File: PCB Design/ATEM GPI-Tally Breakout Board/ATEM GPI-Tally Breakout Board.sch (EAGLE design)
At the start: 22 parts, among them X1 DB25M

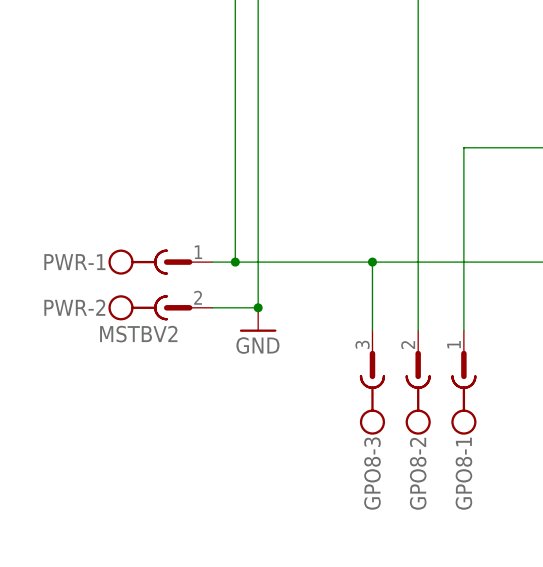
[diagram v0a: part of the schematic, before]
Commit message: Updates for PCBs and more
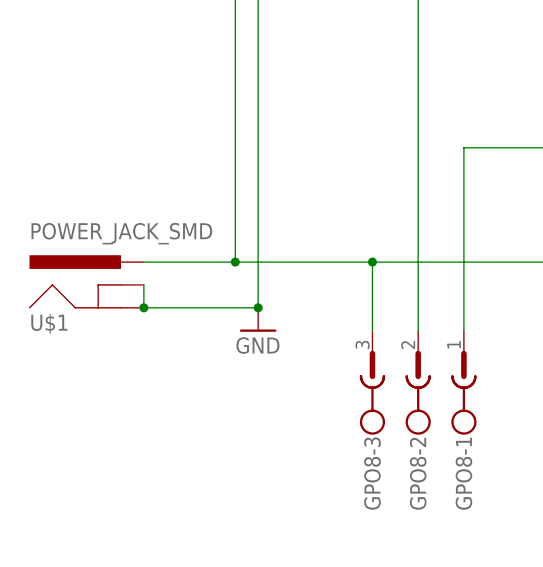
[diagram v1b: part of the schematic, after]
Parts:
- removed PWR: MSTBV2, con-phoenix-508:MSTBV2
- added U$1: POWER_JACK_SMD, SKAARHOJ:POWER_JACK_SMD
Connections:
- net GND: now also U$1.GND, U$1.GNDBREAK; no longer PWR-2.1
- net N$75: now also U$1.PWR; no longer PWR-1.1
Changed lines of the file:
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@@
 <?xml version="1.0" encoding="utf-8"?>
 <!DOCTYPE eagle SYSTEM "eagle.dtd">
-<eagle version="6.1">
+<eagle version="6.2">
 <drawing>
 <settings>
@@
 </variantdefs>
 <classes>
-<class number="0" name="default" width="0" drill="0">
+<class number="0" name="default" width="0.254" drill="0.4064">
+<clearance class="0" value="0.254"/>
 </class>
-<class number="1" name="PWR" width="0.4064" drill="0">
+<class number="1" name="PWR" width="0.8128" drill="0.6096">
 <clearance class="1" value="0.254"/>
 </class>
-<class number="2" name="RELAY LINES" width="0.4064" drill="0">
+<class number="2" name="RELAY LINES" width="0.8128" drill="0.6096">
 <clearance class="2" value="0.254"/>
 </class>
-<class number="3" name="INput lines" width="0" drill="0">
+<class number="3" name="INput lines" width="0.254" drill="0.4064">
 <clearance class="3" value="0.254"/>
 </class>
@@
 <part name="GPO7" library="con-phoenix-508" deviceset="MSTBV3" device="" value="CON1"/>
 <part name="GPO8" library="con-phoenix-508" deviceset="MSTBV3" device="" value="CON1"/>
-<part name="PWR" library="con-phoenix-508" deviceset="MSTBV2" device=""/>
 <part name="GND5" library="SparkFun" deviceset="GND" device=""/>
 <part name="GND1" library="SparkFun" deviceset="GND" device=""/>
@@
 <attribute name="OC_NEWARK" value="69R9845"/>
 </part>
+<part name="U$1" library="SKAARHOJ" deviceset="POWER_JACK_SMD" device=""/>
 </parts>
 <sheets>
@@
 <attribute name="NAME" x="-160.909" y="-19.304" size="1.778" layer="95" rot="R270"/>
 </instance>
-<instance part="PWR" gate="-1" x="-182.88" y="0"/>
-<instance part="PWR" gate="-2" x="-182.88" y="-5.08"/>
 <instance part="GND5" gate="1" x="-172.72" y="-7.62"/>
 <instance part="GND1" gate="1" x="154.94" y="25.4"/>
@@
 <instance part="GPI8" gate="-1" x="-154.94" y="-86.36" rot="R90"/>
 <instance part="GPI8" gate="-2" x="-149.86" y="-86.36" rot="R90"/>
+<instance part="U$1" gate="G$1" x="-185.42" y="-5.08"/>
 </instances>
 <busses>
@@
 <pinref part="GPO1" gate="-2" pin="1"/>
 <wire x1="78.74" y1="-7.62" x2="78.74" y2="33.02" width="0.1524" layer="91"/>
-<pinref part="PWR" gate="-2" pin="1"/>
-<wire x1="-177.8" y1="-5.08" x2="-172.72" y2="-5.08" width="0.1524" layer="91"/>
 <wire x1="-172.72" y1="-5.08" x2="-172.72" y2="33.02" width="0.1524" layer="91"/>
 <pinref part="GND5" gate="1" pin="GND"/>
@@
 <junction x="121.92" y="40.64"/>
 <junction x="78.74" y="33.02"/>
+<wire x1="-185.42" y1="-5.08" x2="-172.72" y2="-5.08" width="0.1524" layer="91"/>
+<pinref part="U$1" gate="G$1" pin="GND"/>
+<pinref part="U$1" gate="G$1" pin="GNDBREAK"/>
+<wire x1="-185.42" y1="-2.54" x2="-185.42" y2="-5.08" width="0.1524" layer="91"/>
+<junction x="-185.42" y="-5.08"/>
 </segment>
 <segment>
@@
 <segment>
 <pinref part="GPO8" gate="-3" pin="1"/>
-<pinref part="PWR" gate="-1" pin="1"/>
-<wire x1="-177.8" y1="0" x2="-175.26" y2="0" width="0.1524" layer="91"/>
 <wire x1="-175.26" y1="0" x2="-160.02" y2="0" width="0.1524" layer="91"/>
 <wire x1="-160.02" y1="0" x2="-160.02" y2="-7.62" width="0.1524" layer="91"/>
@@
 <pinref part="R1" gate="G$1" pin="1"/>
 <wire x1="-175.26" y1="83.82" x2="71.12" y2="83.82" width="0.1524" layer="91"/>
-</segment>
-</net>
+<wire x1="-185.42" y1="0" x2="-175.26" y2="0" width="0.1524" layer="91"/>
+<pinref part="U$1" gate="G$1" pin="PWR"/>
+</segment>
+</net>
